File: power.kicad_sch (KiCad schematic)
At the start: 24 parts

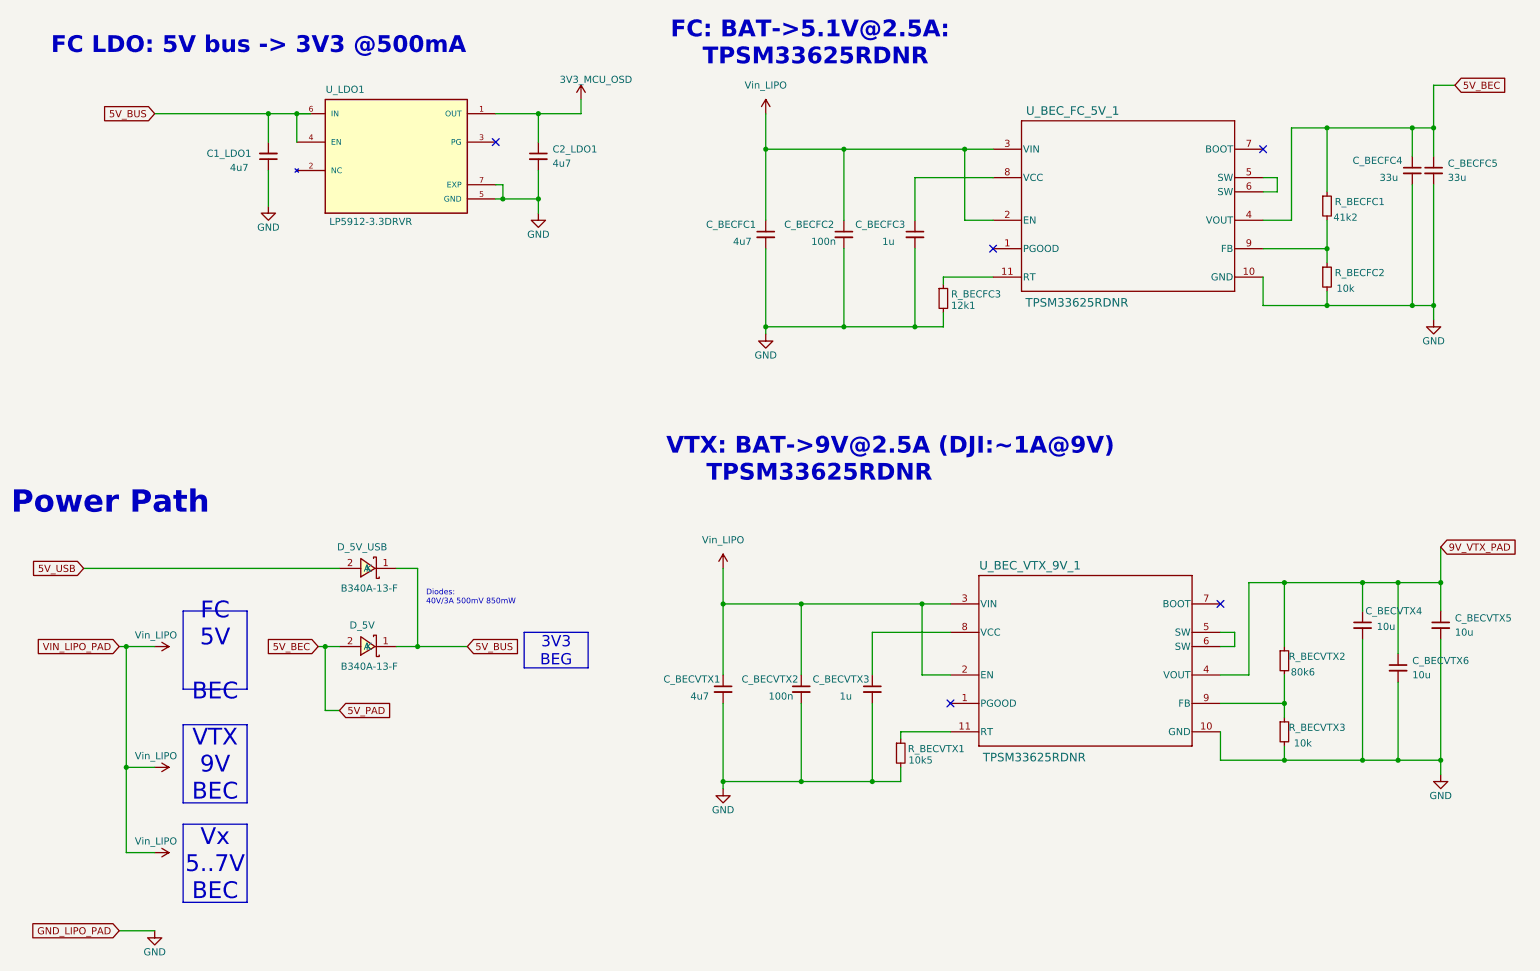
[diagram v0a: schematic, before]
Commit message: regulators
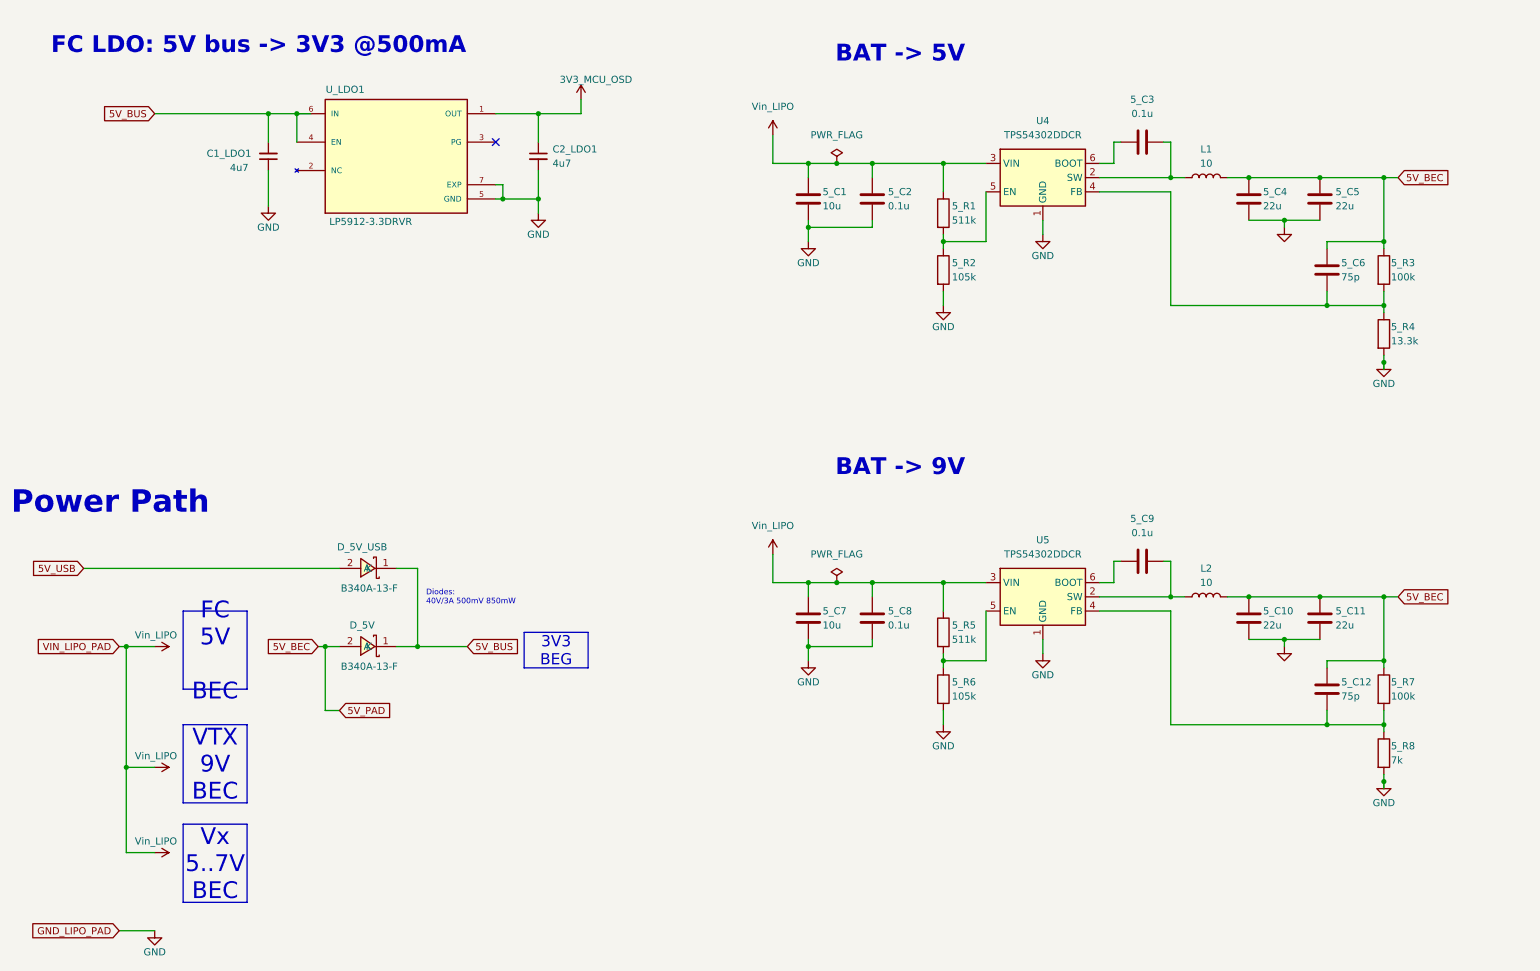
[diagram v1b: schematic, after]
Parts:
- removed C_BECFC1, C_BECVTX1: 4u7, Capacitor_SMD:C_1206_3216Metric, symbol Device:C_Small
- removed C_BECFC2, C_BECVTX2: 100n, Capacitor_SMD:C_1206_3216Metric, symbol Device:C_Small
- removed C_BECFC3, C_BECVTX3: 1u, Capacitor_SMD:C_1206_3216Metric, symbol Device:C_Small
- removed C_BECFC4, C_BECFC5: 33u, Capacitor_SMD:C_1206_3216Metric, symbol Device:C_Small
- removed C_BECVTX4, C_BECVTX5, C_BECVTX6: 10u, Capacitor_SMD:C_1206_3216Metric, symbol Device:C_Small
- removed R_BECFC1: 41k2, Resistor_SMD:R_0402_1005Metric, symbol Device:R_Small
- removed R_BECFC2, R_BECVTX3: 10k, Resistor_SMD:R_0402_1005Metric, symbol Device:R_Small
- removed R_BECFC3: 12k1, Resistor_SMD:R_0402_1005Metric, symbol Device:R_Small
- removed R_BECVTX1: 10k5, Resistor_SMD:R_0402_1005Metric, symbol Device:R_Small
- removed R_BECVTX2: 80k6, Resistor_SMD:R_0402_1005Metric, symbol Device:R_Small
- removed U_BEC_FC_5V_1, U_BEC_VTX_9V_1: TPSM33625RDNR, RDN0011A-MFG, symbol custom_Library:TPSM33625RDNR
- added 5_C1, 5_C7: 10u, Capacitor_SMD:C_0603_1608Metric, symbol Device:C
- added 5_C10, 5_C11, 5_C4, 5_C5: 22u, Capacitor_SMD:C_0805_2012Metric, symbol Device:C
- added 5_C12, 5_C6: 75p, Capacitor_SMD:C_0402_1005Metric, symbol Device:C
- added 5_C2, 5_C3, 5_C8, 5_C9: 0.1u, Capacitor_SMD:C_0402_1005Metric, symbol Device:C
- added 5_R1, 5_R5: 511k, Resistor_SMD:R_0603_1608Metric, symbol Device:R
- added 5_R2, 5_R6: 105k, Resistor_SMD:R_0603_1608Metric, symbol Device:R
- added 5_R3, 5_R7: 100k, Resistor_SMD:R_0603_1608Metric, symbol Device:R
- added 5_R4: 13.3k, Resistor_SMD:R_0402_1005Metric, symbol Device:R
- added 5_R8: 7k, Resistor_SMD:R_0402_1005Metric, symbol Device:R
- added L1, L2: 10, Capacitor_SMD:C_0603_1608Metric, symbol Device:L
- added U4, U5: TPS54302DDCR, Package_TO_SOT_SMD:SOT-23-6, symbol Regulator_Switching:TPS54302
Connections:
- net 5V_BEC: now also 5_C10.1, 5_C11.1, 5_C12.1, 5_C4.1, 5_C5.1, 5_C6.1, 5_R3.1, 5_R7.1, L1.2, L2.2
- net GND: now also 5_C1.2, 5_C10.2, 5_C11.2, 5_C2.2, 5_C4.2, 5_C5.2, 5_C7.2, 5_C8.2, 5_R2.2, 5_R4.2, 5_R6.2, 5_R8.2, U4.1 (GND), U5.1 (GND)
- net Vin_LIPO: now also 5_C1.1, 5_C2.1, 5_C7.1, 5_C8.1, 5_R1.1, 5_R5.1, U4.3 (VIN), U5.3 (VIN)
- new net: 5_C3.2, L1.1, U4.2 (SW)
- new net: 5_C6.2, 5_R3.2, 5_R4.1, U4.4 (FB)
- new net: 5_R1.2, 5_R2.1, U4.5 (EN)
- new net: 5_C3.1, U4.6 (BOOT)
- new net: 5_C9.2, L2.1, U5.2 (SW)
- new net: 5_C12.2, 5_R7.2, 5_R8.1, U5.4 (FB)
- new net: 5_R5.2, 5_R6.1, U5.5 (EN)
- new net: 5_C9.1, U5.6 (BOOT)
- no-connect marks 5 -> 1
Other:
- note added: "BAT -> 5V"
- note added: "BAT -> 9V"
- note removed: "FC: BAT->5.1V@2.5A: TPSM33625RDNR"
- note removed: "VTX: BAT->9V@2.5A (DJI:~1A@9V) TPSM33625RDNR"
